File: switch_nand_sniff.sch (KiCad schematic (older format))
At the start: 7 parts, among them P1 CONN_02X15, P2 CONN_02X15, P3 CONN_01X02, P4 CONN_01X02

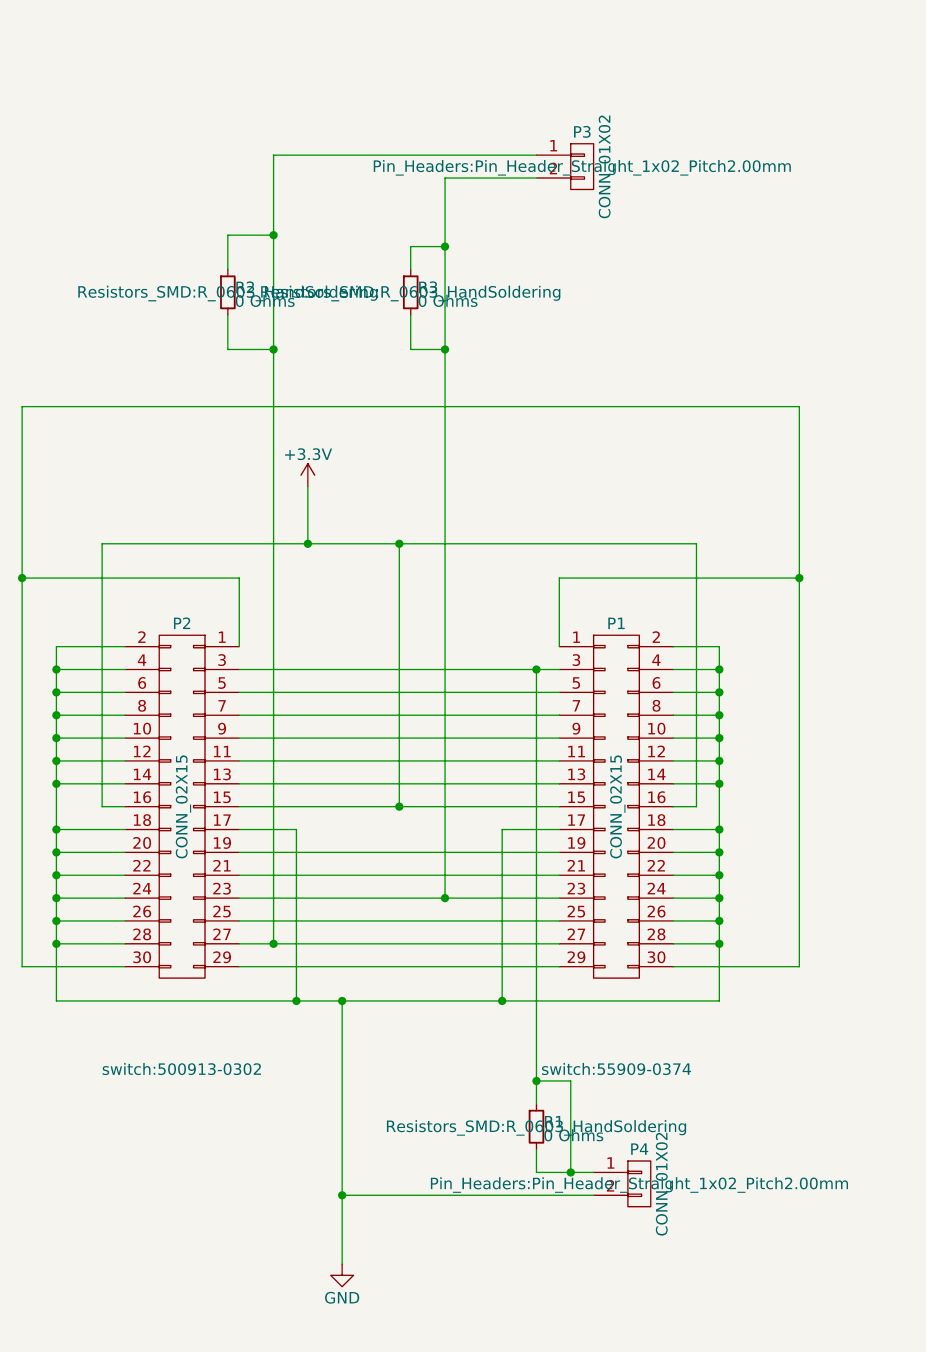
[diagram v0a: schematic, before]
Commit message: Add sip-8. staging before rollback to find resistor desired.
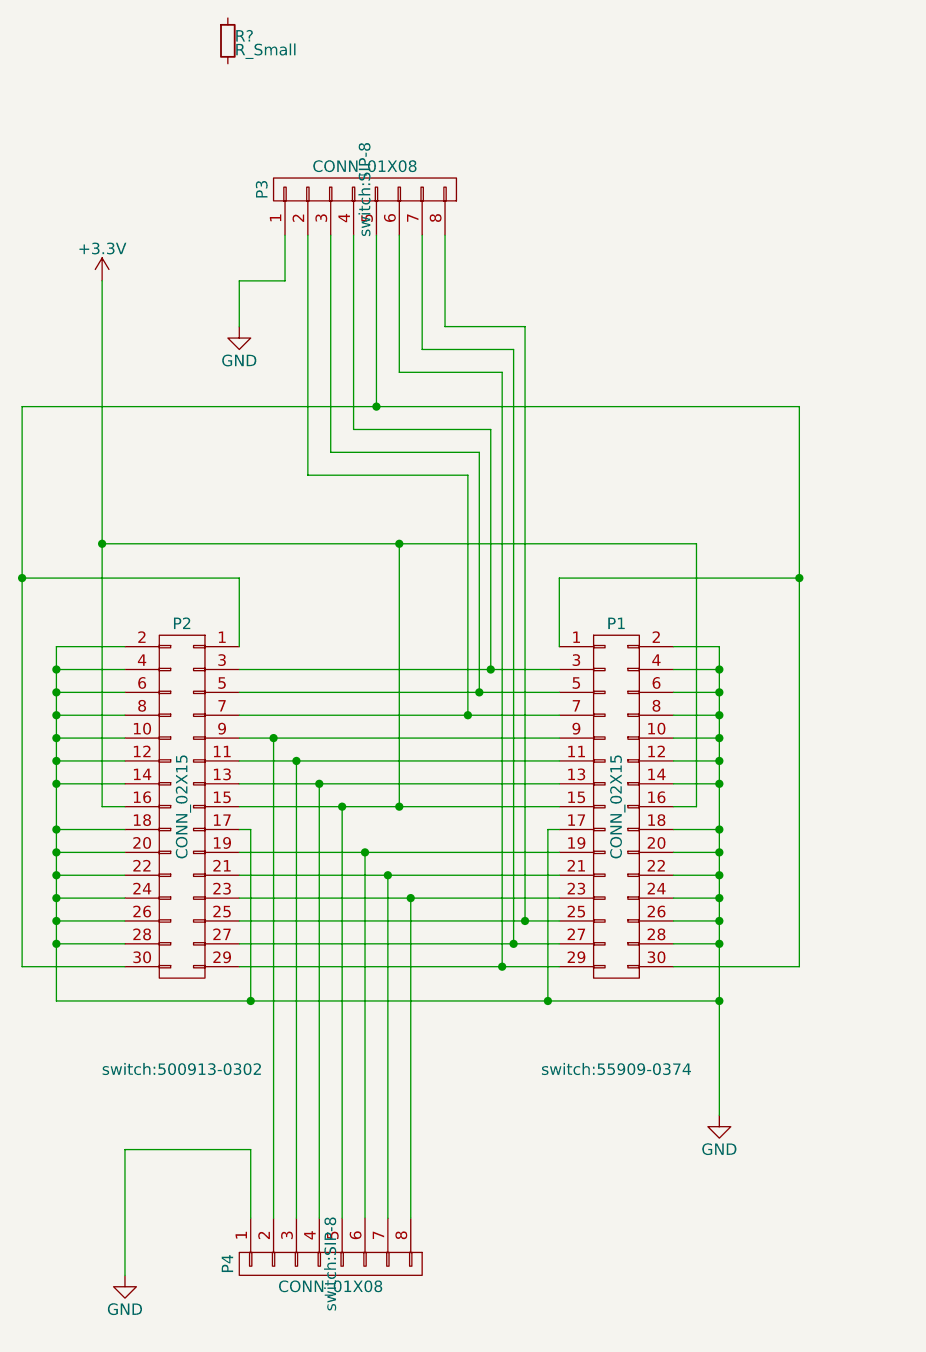
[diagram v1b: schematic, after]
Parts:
- removed P3, P4: CONN_01X02, Pin_Headers:Pin_Header_Straight_1x02_Pitch2.00mm, symbol CONN_01X02
- removed R1, R2, R3: 0 Ohms, Resistors_SMD:R_0603_HandSoldering, symbol R_Small
- added P3, P4: CONN_01X08, switch:SIP-8, symbol CONN_01X08
- added R?: R_Small, symbol R_Small
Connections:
- net +3V3: now also P4.5 (P5)
- net GND: now also P3.1 (P1), P4.1 (P1)
- net at P1.1 (P1), P1.30 (P30), P2.1 (P1)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: now also P3.5 (P5)
- net at P1.11 (P11), P2.11 (P11): now also P4.3 (P3)
- net at P1.13 (P13), P2.13 (P13): now also P4.4 (P4)
- net at P1.19 (P19), P2.19 (P19): now also P4.6 (P6)
- net at P1.21 (P21), P2.21 (P21): now also P4.7 (P7)
- net at P1.23 (P23), P2.23 (P23): now also P4.8 (P8)
- net at P1.25 (P25), P2.25 (P25): now also P3.8 (P8)
- net at P1.27 (P27), P2.27 (P27): now also P3.7 (P7)
- net at P1.29 (P29), P2.29 (P29): now also P3.6 (P6)
- net at P1.3 (P3), P2.3 (P3): now also P3.4 (P4)
- net at P1.5 (P5), P2.5 (P5): now also P3.3 (P3)
- net at P1.7 (P7), P2.7 (P7): now also P3.2 (P2)
- net at P1.9 (P9), P2.9 (P9): now also P4.2 (P2)
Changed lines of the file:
@@
 	3300 3400 4700 3400
 Wire Wire Line
-	4700 3500 3300 3500
+	3300 3500 4700 3500
 Wire Wire Line
 	3300 3600 4700 3600
@@
 	4700 4200 3300 4200
 Wire Wire Line
-	3300 4300 4700 4300
-Wire Wire Line
 	3300 4400 4700 4400
 Wire Wire Line
@@
 	3300 4600 4700 4600
 Wire Wire Line
-	4700 3200 4700 2900
-Wire Wire Line
-	4700 2900 5750 2900
-Wire Wire Line
 	5750 2150 5750 4600
 Wire Wire Line
@@
 	5200 3200 5400 3200
 Wire Wire Line
-	5400 3200 5400 4750
+	5400 3200 5400 5250
 Wire Wire Line
 	5400 4500 5200 4500
@@
 	3300 3900 4700 3900
 Wire Wire Line
-	2800 3900 2700 3900
-Wire Wire Line
-	2700 3900 2700 2750
+	2700 3900 2800 3900
+Wire Wire Line
+	2700 1600 2700 3900
 Wire Wire Line
 	2700 2750 5300 2750
@@
 Connection ~ 2500 4500
 Wire Wire Line
-	3300 4000 3550 4000
-Wire Wire Line
-	3550 4000 3550 4750
-Connection ~ 3550 4750
-Wire Wire Line
-	4700 4000 4450 4000
-Wire Wire Line
-	4450 4000 4450 4750
-Connection ~ 4450 4750
-$Comp
-L GND #PWR01
-U 1 1 599BAC3C
-P 3750 5900
-F 0 "#PWR01" H 3750 5650 50  0001 C CNN
-F 1 "GND" H 3750 5750 50  0000 C CNN
-F 2 "" H 3750 5900 50  0000 C CNN
-F 3 "" H 3750 5900 50  0000 C CNN
-	1    3750 5900
-	1    0    0    -1
-$EndComp
-Wire Wire Line
-	3750 4750 3750 5900
-Connection ~ 3750 4750
+	3300 4000 3350 4000
+Wire Wire Line
+	3350 4000 3350 4750
+Connection ~ 3350 4750
+Wire Wire Line
+	4700 4000 4650 4000
+Wire Wire Line
+	4650 4000 4650 4750
+Connection ~ 4650 4750
+Connection ~ 5400 4750
 Connection ~ 5400 4000
 Connection ~ 5400 3800
 $Comp
-L +3.3V #PWR02
+L +3.3V #PWR01
 U 1 1 599BADE4
-P 3600 2500
-F 0 "#PWR02" H 3600 2350 50  0001 C CNN
-F 1 "+3.3V" H 3600 2640 50  0000 C CNN
-F 2 "" H 3600 2500 50  0000 C CNN
-F 3 "" H 3600 2500 50  0000 C CNN
-	1    3600 2500
-	1    0    0    -1
-$EndComp
-Wire Wire Line
-	3600 2500 3600 2750
-Connection ~ 3600 2750
-Wire Wire Line
-	5750 2150 2350 2150
+P 2700 1600
+F 0 "#PWR01" H 2700 1450 50  0001 C CNN
+F 1 "+3.3V" H 2700 1740 50  0000 C CNN
+F 2 "" H 2700 1600 50  0000 C CNN
+F 3 "" H 2700 1600 50  0000 C CNN
+	1    2700 1600
+	1    0    0    -1
+$EndComp
+Connection ~ 2700 2750
+Wire Wire Line
+	2350 2150 5750 2150
 Connection ~ 2350 2900
+$Comp
+L GND #PWR02
+U 1 1 59AB99FC
+P 5400 5250
+F 0 "#PWR02" H 5400 5000 50  0001 C CNN
+F 1 "GND" H 5400 5100 50  0000 C CNN
+F 2 "" H 5400 5250 50  0000 C CNN
+F 3 "" H 5400 5250 50  0000 C CNN
+	1    5400 5250
+	1    0    0    -1
+$EndComp
+$Comp
+L CONN_01X08 P3
+U 1 1 59AB9B20
+P 3850 1200
+F 0 "P3" H 3850 1650 50  0000 C CNN
+F 1 "CONN_01X08" V 3950 1200 50  0000 C CNN
+F 2 "switch:SIP-8" H 3850 1200 50  0000 C CNN
+F 3 "" H 3850 1200 50  0000 C CNN
+	1    3850 1200
+	0    -1   -1   0
+$EndComp
+$Comp
+L CONN_01X08 P4
+U 1 1 59AB9BC3
+P 3700 5900
+F 0 "P4" H 3700 6350 50  0000 C CNN
+F 1 "CONN_01X08" V 3800 5900 50  0000 C CNN
+F 2 "switch:SIP-8" H 3700 5900 50  0000 C CNN
+F 3 "" H 3700 5900 50  0000 C CNN
+	1    3700 5900
+	0    -1   1    0
+$EndComp
+Wire Wire Line
+	3300 4300 4700 4300
+Wire Wire Line
+	4550 4400 4550 1800
+Wire Wire Line
+	4550 1800 4200 1800
+Wire Wire Line
+	4200 1800 4200 1400
+Connection ~ 4550 4400
+Wire Wire Line
+	4500 4500 4500 1900
+Wire Wire Line
+	4500 1900 4100 1900
+Wire Wire Line
+	4100 1900 4100 1400
+Connection ~ 4500 4500
+Wire Wire Line
+	4450 4600 4450 2000
+Wire Wire Line
+	4450 2000 4000 2000
+Wire Wire Line
+	4000 2000 4000 1400
+Connection ~ 4450 4600
+Wire Wire Line
+	3900 1400 3900 2150
+Connection ~ 3900 2150
+Wire Wire Line
+	4400 3300 4400 2250
+Connection ~ 4400 3300
+Wire Wire Line
+	4400 2250 3800 2250
 Connection ~ 5750 2900
-$Comp
-L CONN_01X02 P3
-U 1 1 599D1913
-P 4800 1100
-F 0 "P3" H 4800 1250 50  0000 C CNN
-F 1 "CONN_01X02" V 4900 1100 50  0000 C CNN
-F 2 "Pin_Headers:Pin_Header_Straight_1x02_Pitch2.00mm" H 4800 1100 50  0000 C CNN
-F 3 "" H 4800 1100 50  0000 C CNN
-	1    4800 1100
-	1    0    0    -1
-$EndComp
-$Comp
-L CONN_01X02 P4
-U 1 1 599D19F1
-P 5050 5550
-F 0 "P4" H 5050 5700 50  0000 C CNN
-F 1 "CONN_01X02" V 5150 5550 50  0000 C CNN
-F 2 "Pin_Headers:Pin_Header_Straight_1x02_Pitch2.00mm" H 5050 5550 50  0000 C CNN
-F 3 "" H 5050 5550 50  0000 C CNN
-	1    5050 5550
-	1    0    0    -1
-$EndComp
-Wire Wire Line
-	4600 5500 4850 5500
-Connection ~ 4600 3300
-Wire Wire Line
-	3750 5600 4850 5600
-Connection ~ 3750 5600
-Connection ~ 3450 4500
-Connection ~ 4200 4300
-$Comp
-L R_Small R1
-U 1 1 599D1FA2
-P 4600 5300
-F 0 "R1" H 4630 5320 50  0000 L CNN
-F 1 "0 Ohms" H 4630 5260 50  0000 L CNN
-F 2 "Resistors_SMD:R_0603_HandSoldering" H 4600 5300 50  0000 C CNN
-F 3 "" H 4600 5300 50  0000 C CNN
-	1    4600 5300
-	1    0    0    -1
-$EndComp
-Wire Wire Line
-	4600 5400 4600 5500
-Wire Wire Line
-	4600 3300 4600 5200
-Wire Wire Line
-	4600 5100 4750 5100
-Wire Wire Line
-	4750 5100 4750 5500
-Connection ~ 4750 5500
-Connection ~ 4600 5100
-Wire Wire Line
-	4200 4300 4200 1150
-Wire Wire Line
-	4200 1150 4600 1150
-Wire Wire Line
-	3450 4500 3450 1050
-Wire Wire Line
-	3450 1050 4600 1050
-$Comp
-L R_Small R3
-U 1 1 599DE5B4
-P 4050 1650
-F 0 "R3" H 4080 1670 50  0000 L CNN
-F 1 "0 Ohms" H 4080 1610 50  0000 L CNN
-F 2 "Resistors_SMD:R_0603_HandSoldering" H 4050 1650 50  0000 C CNN
-F 3 "" H 4050 1650 50  0000 C CNN
-	1    4050 1650
-	1    0    0    -1
-$EndComp
-$Comp
-L R_Small R2
-U 1 1 599DE684
-P 3250 1650
-F 0 "R2" H 3280 1670 50  0000 L CNN
-F 1 "0 Ohms" H 3280 1610 50  0000 L CNN
-F 2 "Resistors_SMD:R_0603_HandSoldering" H 3250 1650 50  0000 C CNN
-F 3 "" H 3250 1650 50  0000 C CNN
-	1    3250 1650
-	1    0    0    -1
-$EndComp
-Wire Wire Line
-	4050 1550 4050 1450
-Wire Wire Line
-	4050 1450 4200 1450
-Connection ~ 4200 1450
-Wire Wire Line
-	4050 1750 4050 1900
-Wire Wire Line
-	4050 1900 4200 1900
-Connection ~ 4200 1900
-Wire Wire Line
-	3250 1550 3250 1400
-Wire Wire Line
-	3250 1400 3450 1400
-Connection ~ 3450 1400
-Wire Wire Line
-	3250 1750 3250 1900
-Wire Wire Line
-	3250 1900 3450 1900
-Connection ~ 3450 1900
+Wire Wire Line
+	4700 2900 4700 3200
+Wire Wire Line
+	4700 2900 5750 2900
+Wire Wire Line
+	3800 2250 3800 1400
+Wire Wire Line
+	3700 1400 3700 2350
+Wire Wire Line
+	3700 2350 4350 2350
+Wire Wire Line
+	4350 2350 4350 3400
+Connection ~ 4350 3400
+Wire Wire Line
+	3600 1400 3600 2450
+Wire Wire Line
+	3600 2450 4300 2450
+Wire Wire Line
+	4300 2450 4300 3500
+Connection ~ 4300 3500
+$Comp
+L GND #PWR03
+U 1 1 59ABAC3D
+P 3300 1800
+F 0 "#PWR03" H 3300 1550 50  0001 C CNN
+F 1 "GND" H 3300 1650 50  0000 C CNN
+F 2 "" H 3300 1800 50  0000 C CNN
+F 3 "" H 3300 1800 50  0000 C CNN
+	1    3300 1800
+	1    0    0    -1
+$EndComp
+Wire Wire Line
+	3500 1400 3500 1600
+Wire Wire Line
+	3500 1600 3300 1600
+Wire Wire Line
+	3300 1600 3300 1800
+$Comp
+L GND #PWR04
+U 1 1 59ABAD1B
+P 2800 5950
+F 0 "#PWR04" H 2800 5700 50  0001 C CNN
+F 1 "GND" H 2800 5800 50  0000 C CNN
+F 2 "" H 2800 5950 50  0000 C CNN
+F 3 "" H 2800 5950 50  0000 C CNN
+	1    2800 5950
+	1    0    0    -1
+$EndComp
+Wire Wire Line
+	3350 5700 3350 5400
+Wire Wire Line
+	3350 5400 2800 5400
+Wire Wire Line
+	2800 5400 2800 5950
+Wire Wire Line
+	3450 5700 3450 3600
+Connection ~ 3450 3600
+Wire Wire Line
+	3550 5700 3550 3700
+Connection ~ 3550 3700
+Wire Wire Line
+	3650 5700 3650 3800
+Connection ~ 3650 3800
+Wire Wire Line
+	3750 5700 3750 3900
+Connection ~ 3750 3900
+Wire Wire Line
+	3850 5700 3850 4100
+Connection ~ 3850 4100
+Wire Wire Line
+	3950 5700 3950 4200
+Connection ~ 3950 4200
+Wire Wire Line
+	4050 5700 4050 4300
+Connection ~ 4050 4300
+$Comp
+L R_Small R?
+U 1 1 59ABBED3
+P 3250 550
+F 0 "R?" H 3280 570 50  0000 L CNN
+F 1 "R_Small" H 3280 510 50  0000 L CNN
+F 2 "" H 3250 550 50  0000 C CNN
+F 3 "" H 3250 550 50  0000 C CNN
+	1    3250 550
+	1    0    0    -1
+$EndComp
 $EndSCHEMATC
